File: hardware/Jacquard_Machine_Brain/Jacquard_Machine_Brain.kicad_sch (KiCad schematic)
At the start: 63 parts, among them J1 Terminal Block, J15 USB_A, J2 Conn_01x08, J200 WIZnet_J1B1211CCD_RJ45, J3 JST-SH 01x04, J4 Conn_01x02, J5 Conn_01x02, J6 Conn_02x08_Odd_Even, U1 R-78E5.0-1.0, U10 74AHCT1G125, U2 Teensy4.1, U3 74AHCT1G125, U4 74AHCT1G125, U6 AO4882, U7 74AHCT1G125, U8 74AHCT1G125, U9 PCA9306D

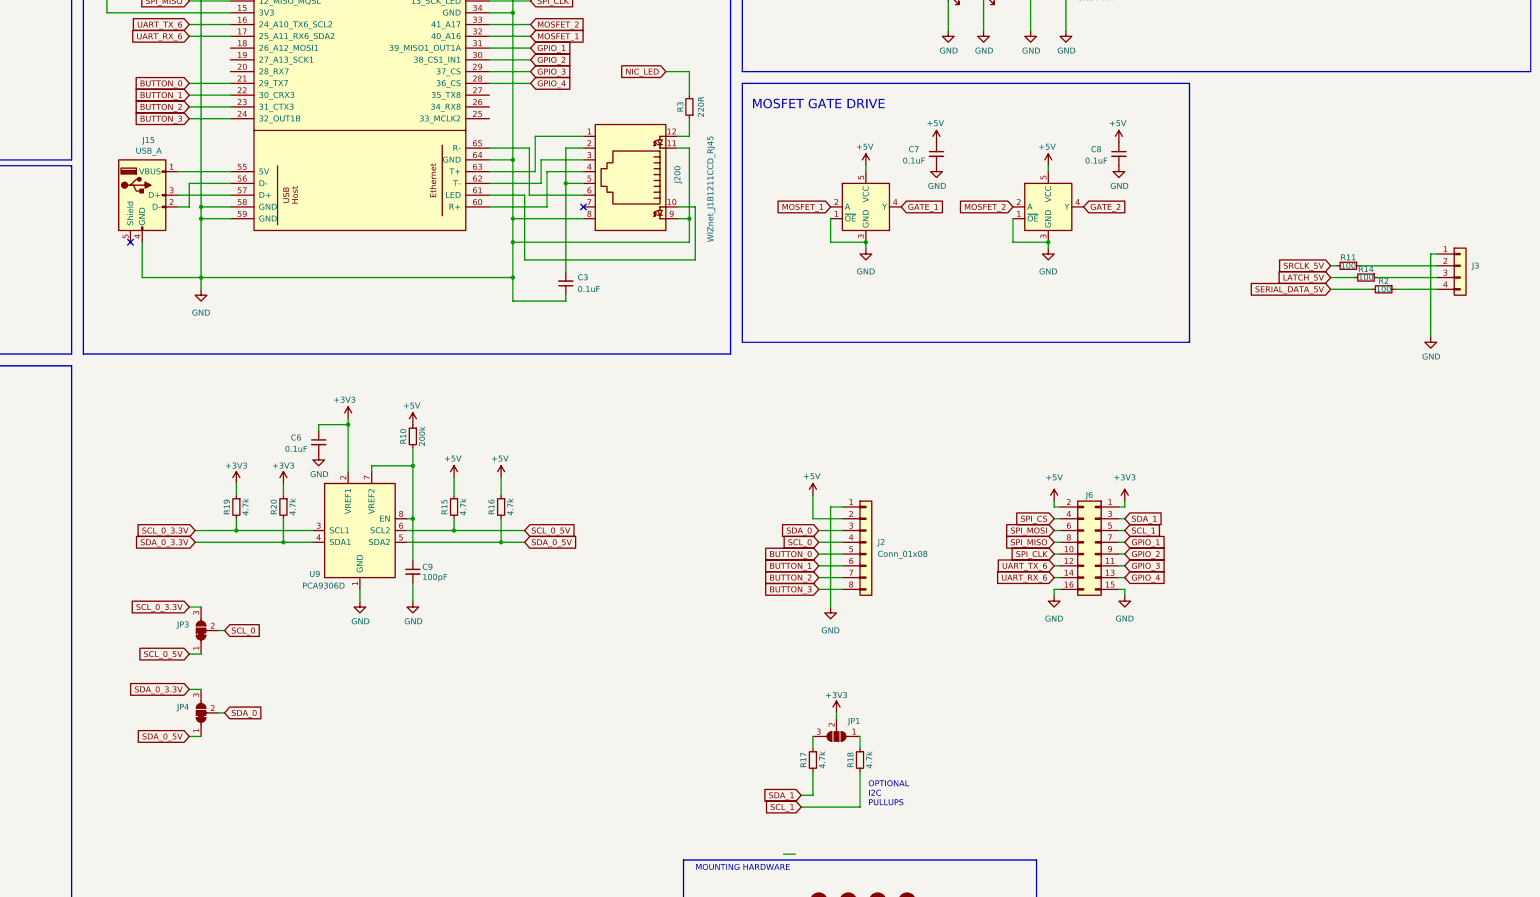
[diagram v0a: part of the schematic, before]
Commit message: PCB Wrap up
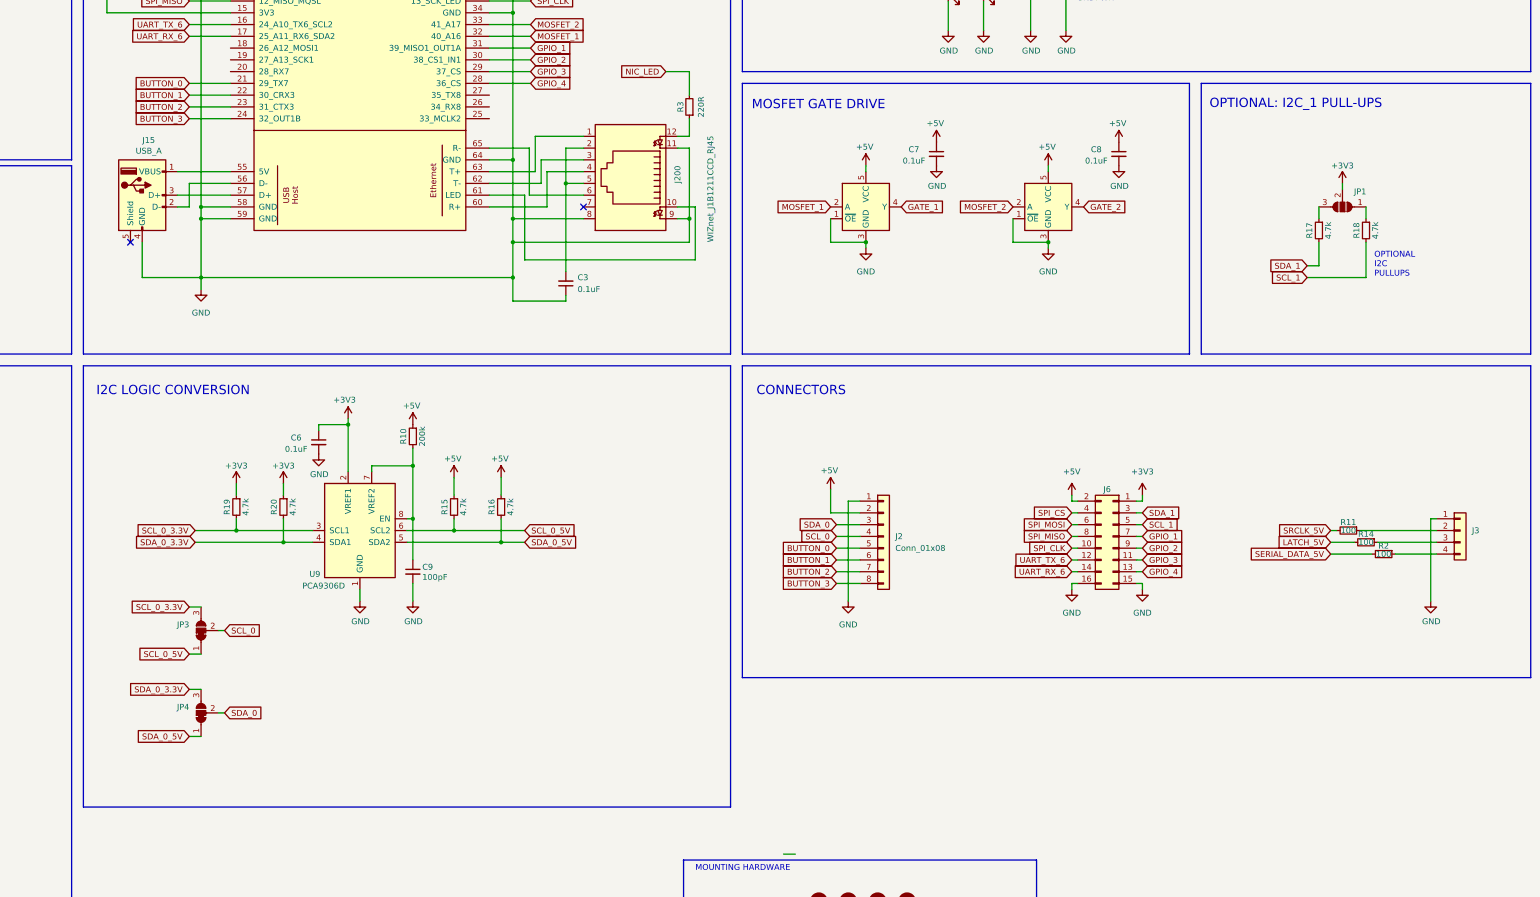
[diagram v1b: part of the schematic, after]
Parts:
- C2: LCSC C50254 -> C377773
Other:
- note added: "CONNECTORS"
- note added: "I2C LOGIC CONVERSION"
- note added: "OPTIONAL: I2C_1 PULL-UPS"
- company: Meow Wolf -> Daniel Bornhorst
- title: (none) -> Jacuard Machine Brain
- moved on the sheet: J2, J3, J6, JP1, R11, R14, R17, R18, R2
